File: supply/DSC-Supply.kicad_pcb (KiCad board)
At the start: 2 copper layers, 160 x 100 mm, 23 parts, among them IC1 LM2611, IC2 TPS76933, IC3 TPS76901, IC4 TPS72301

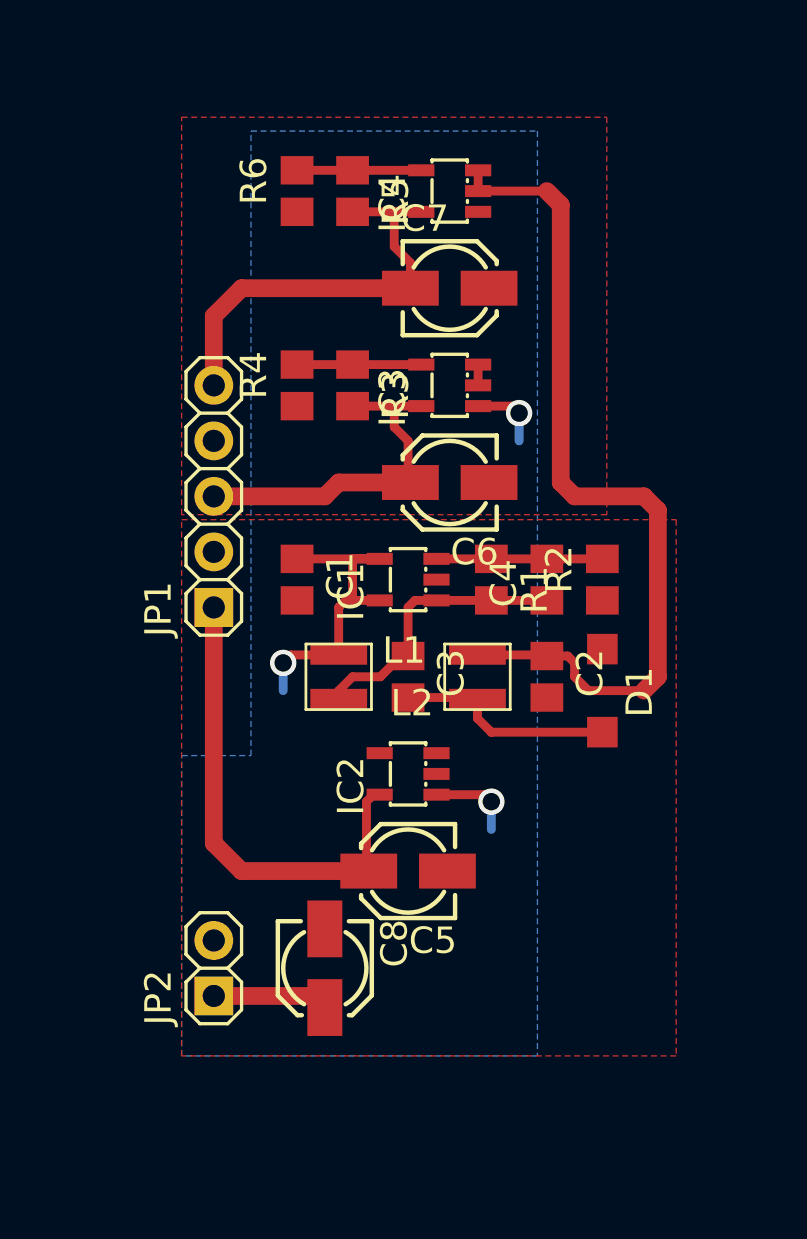
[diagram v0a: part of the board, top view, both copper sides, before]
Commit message: finished PCB v1
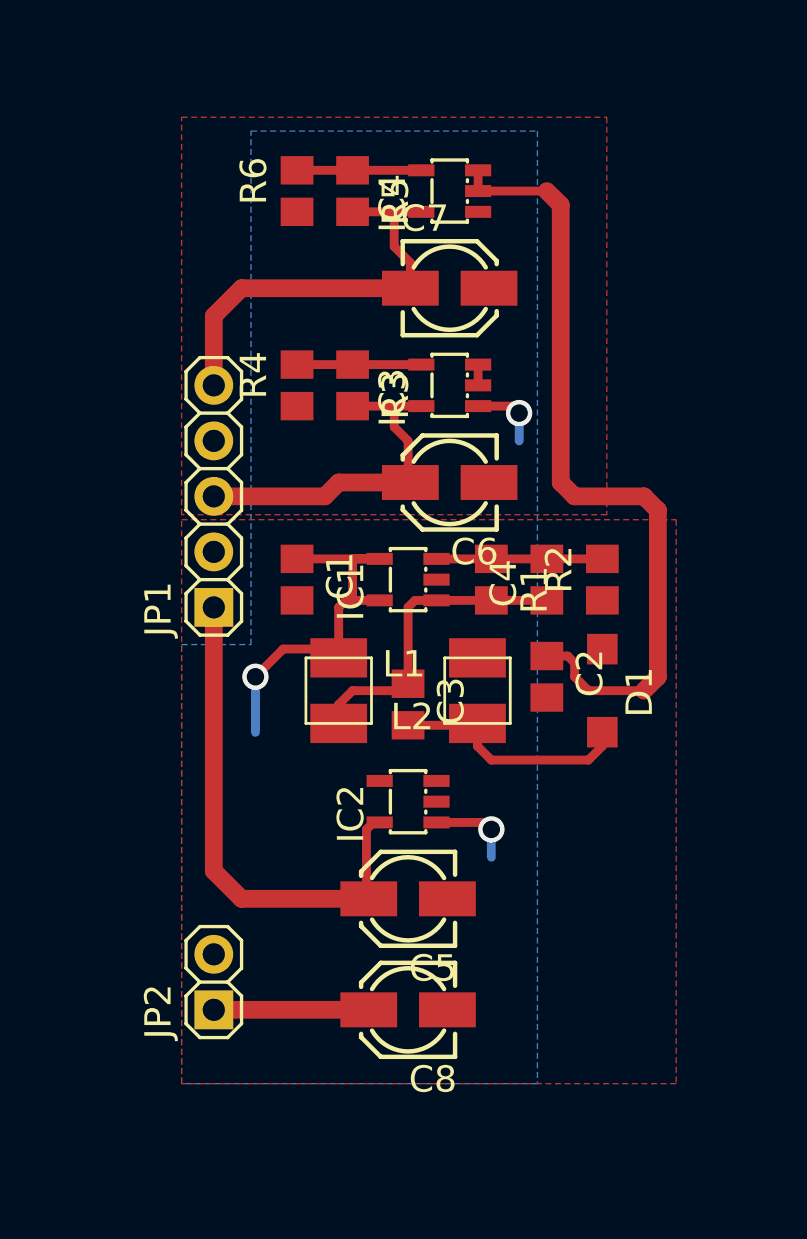
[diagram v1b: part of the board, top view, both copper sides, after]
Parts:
- moved C8 4.26 mm to (123.7, 136.0), turned to 180 degrees
- moved C5 1.27 mm to (123.7, 130.9)
- moved C3 1.27 mm to (123.7, 122.0)
- moved IC2 1.27 mm to (123.7, 126.4)
- moved JP2 0.64 mm to (114.9, 134.7)
- moved L1 0.64 mm to (120.6, 121.3)
- moved L2 0.64 mm to (126.9, 121.3)
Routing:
- net +5V: track 28.0 -> 32.6 mm
- net -5V: track 39.9 -> 36.7 mm
- net Net-(C3-Pad1): track 12.9 -> 14.6 mm
- net +3V3D: track 22.4 -> 23.6 mm
- net Net-(C3-Pad2): track 10.1 -> 11.1 mm
